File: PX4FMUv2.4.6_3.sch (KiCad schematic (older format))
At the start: 5 parts, among them J301 47346-0001, U302 NUF2042XV6

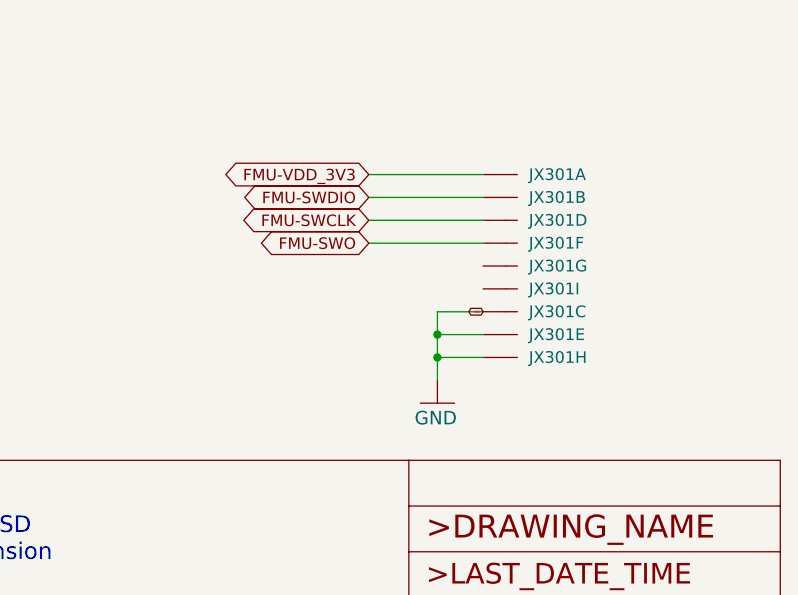
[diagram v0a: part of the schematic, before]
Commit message: removed more things
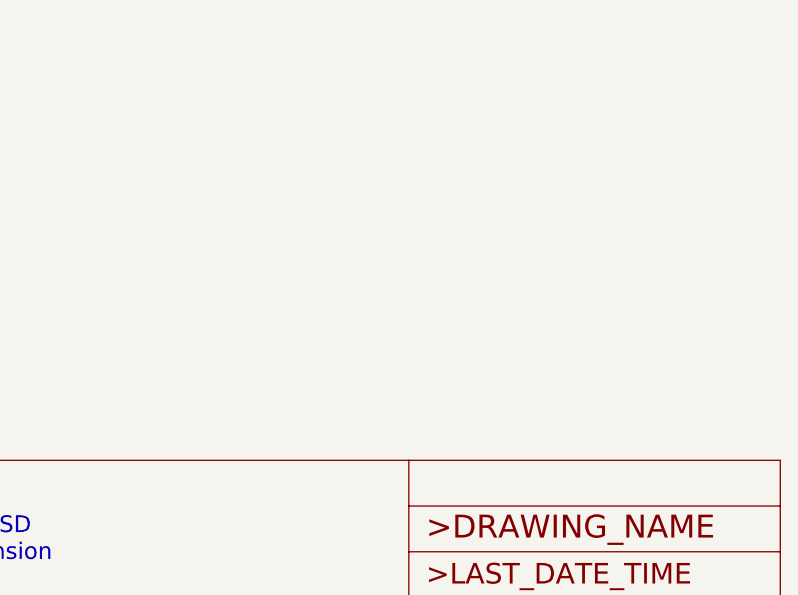
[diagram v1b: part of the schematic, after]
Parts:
- removed JX301: ARM_MINI_JTAG-SMT, PX4FMUv2.4.6:FTSH-105-01-XXX-DV-K, symbol PX4FMUv2.4.6-eagle-import:ARM_MINI_JTAG-SMT
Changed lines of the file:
@@
 $EndDescr
-Wire Wire Line
-	9700 5100 9200 5100
-Text GLabel 9200 5100 0    50   BiDi ~ 0
-FMU-SWDIO
 Wire Wire Line
 	3000 1200 3000 1300
@@
 Text GLabel 4650 1900 0    10   BiDi ~ 0
 GND
-Wire Wire Line
-	9700 5600 9500 5600
-Wire Wire Line
-	9500 5600 9500 5700
-Wire Wire Line
-	9500 5700 9500 5800
-Wire Wire Line
-	9500 5800 9500 5900
-Wire Wire Line
-	9700 5700 9500 5700
-Wire Wire Line
-	9500 5800 9700 5800
-Connection ~ 9500 5700
-Connection ~ 9500 5800
-Text GLabel 9700 5600 0    10   BiDi ~ 0
-GND
-Wire Wire Line
-	9700 5000 9200 5000
-Text GLabel 9200 5000 0    50   BiDi ~ 0
-FMU-VDD_3V3
 Wire Wire Line
 	6600 1200 6800 1200
@@
 Text GLabel 6700 1900 0    50   BiDi ~ 0
 FMU-I2C2_SDA
-Wire Wire Line
-	9700 5300 9200 5300
-Text GLabel 9200 5300 0    50   BiDi ~ 0
-FMU-SWO
-Wire Wire Line
-	9700 5200 9200 5200
-Text GLabel 9200 5200 0    50   BiDi ~ 0
-FMU-SWCLK
 $Comp
 L PX4FMUv2.4.6-eagle-import:A4L-LOC #FRAME6
@@
 	1    0    0    -1
 $EndComp
-$Comp
-L PX4FMUv2.4.6-eagle-import:GND #GND16
-U 1 0 8316678299D4D269
-P 9500 6000
-AR Path="/8316678299D4D269" Ref="#GND16"  Part="1"
-AR Path="/5C109013/8316678299D4D269" Ref="#GND016"  Part="1"
-F 0 "#GND016" H 9500 6000 50  0001 C CNN
-F 1 "GND" H 9400 5900 59  0000 L BNN
-F 2 "" H 9500 6000 50  0001 C CNN
-F 3 "" H 9500 6000 50  0001 C CNN
-	1    9500 6000
-	1    0    0    -1
-$EndComp
-$Comp
-L PX4FMUv2.4.6-eagle-import:ARM_MINI_JTAG-SMT JX301
-U 1 0 F99DB6D9CEB5AE7F
-P 9800 5000
-AR Path="/F99DB6D9CEB5AE7F" Ref="JX301"  Part="1"
-AR Path="/5C109013/F99DB6D9CEB5AE7F" Ref="JX301"  Part="1"
-F 0 "JX301" H 9900 4970 51  0000 L BNN
-F 1 "ARM_MINI_JTAG-SMT" H 9770 5055 59  0001 L BNN
-F 2 "PX4FMUv2.4.6:FTSH-105-01-XXX-DV-K" H 9800 5000 50  0001 C CNN
-F 3 "" H 9800 5000 50  0001 C CNN
-	1    9800 5000
-	1    0    0    -1
-$EndComp
-$Comp
-L PX4FMUv2.4.6-eagle-import:ARM_MINI_JTAG-SMT JX301
-U 2 0 F99DB6D9CEB5AE73
-P 9800 5100
-AR Path="/F99DB6D9CEB5AE73" Ref="JX301"  Part="2"
-AR Path="/5C109013/F99DB6D9CEB5AE73" Ref="JX301"  Part="2"
-F 0 "JX301" H 9900 5070 51  0000 L BNN
-F 1 "ARM_MINI_JTAG-SMT" H 9770 5155 59  0001 L BNN
-F 2 "PX4FMUv2.4.6:FTSH-105-01-XXX-DV-K" H 9800 5100 50  0001 C CNN
-F 3 "" H 9800 5100 50  0001 C CNN
-	2    9800 5100
-	1    0    0    -1
-$EndComp
-$Comp
-L PX4FMUv2.4.6-eagle-import:ARM_MINI_JTAG-SMT JX301
-U 3 0 F99DB6D9CEB5AE77
-P 9800 5600
-AR Path="/F99DB6D9CEB5AE77" Ref="JX301"  Part="3"
-AR Path="/5C109013/F99DB6D9CEB5AE77" Ref="JX301"  Part="3"
-F 0 "JX301" H 9900 5570 51  0000 L BNN
-F 1 "ARM_MINI_JTAG-SMT" H 9770 5655 59  0001 L BNN
-F 2 "PX4FMUv2.4.6:FTSH-105-01-XXX-DV-K" H 9800 5600 50  0001 C CNN
-F 3 "" H 9800 5600 50  0001 C CNN
-	3    9800 5600
-	1    0    0    -1
-$EndComp
-$Comp
-L PX4FMUv2.4.6-eagle-import:ARM_MINI_JTAG-SMT JX301
-U 4 0 F99DB6D9CEB5AE6B
-P 9800 5200
-AR Path="/F99DB6D9CEB5AE6B" Ref="JX301"  Part="4"
-AR Path="/5C109013/F99DB6D9CEB5AE6B" Ref="JX301"  Part="4"
-F 0 "JX301" H 9900 5170 51  0000 L BNN
-F 1 "ARM_MINI_JTAG-SMT" H 9770 5255 59  0001 L BNN
-F 2 "PX4FMUv2.4.6:FTSH-105-01-XXX-DV-K" H 9800 5200 50  0001 C CNN
-F 3 "" H 9800 5200 50  0001 C CNN
-	4    9800 5200
-	1    0    0    -1
-$EndComp
-$Comp
-L PX4FMUv2.4.6-eagle-import:ARM_MINI_JTAG-SMT JX301
-U 5 0 F99DB6D9CEB5AE6F
-P 9800 5700
-AR Path="/F99DB6D9CEB5AE6F" Ref="JX301"  Part="5"
-AR Path="/5C109013/F99DB6D9CEB5AE6F" Ref="JX301"  Part="5"
-F 0 "JX301" H 9900 5670 51  0000 L BNN
-F 1 "ARM_MINI_JTAG-SMT" H 9770 5755 59  0001 L BNN
-F 2 "PX4FMUv2.4.6:FTSH-105-01-XXX-DV-K" H 9800 5700 50  0001 C CNN
-F 3 "" H 9800 5700 50  0001 C CNN
-	5    9800 5700
-	1    0    0    -1
-$EndComp
-$Comp
-L PX4FMUv2.4.6-eagle-import:ARM_MINI_JTAG-SMT JX301
-U 6 0 F99DB6D9CEB5AE63
-P 9800 5300
-AR Path="/F99DB6D9CEB5AE63" Ref="JX301"  Part="6"
-AR Path="/5C109013/F99DB6D9CEB5AE63" Ref="JX301"  Part="6"
-F 0 "JX301" H 9900 5270 51  0000 L BNN
-F 1 "ARM_MINI_JTAG-SMT" H 9770 5355 59  0001 L BNN
-F 2 "PX4FMUv2.4.6:FTSH-105-01-XXX-DV-K" H 9800 5300 50  0001 C CNN
-F 3 "" H 9800 5300 50  0001 C CNN
-	6    9800 5300
-	1    0    0    -1
-$EndComp
-$Comp
-L PX4FMUv2.4.6-eagle-import:ARM_MINI_JTAG-SMT JX301
-U 7 0 F99DB6D9CEB5AE67
-P 9800 5400
-AR Path="/F99DB6D9CEB5AE67" Ref="JX301"  Part="7"
-AR Path="/5C109013/F99DB6D9CEB5AE67" Ref="JX301"  Part="7"
-F 0 "JX301" H 9900 5370 51  0000 L BNN
-F 1 "ARM_MINI_JTAG-SMT" H 9770 5455 59  0001 L BNN
-F 2 "PX4FMUv2.4.6:FTSH-105-01-XXX-DV-K" H 9800 5400 50  0001 C CNN
-F 3 "" H 9800 5400 50  0001 C CNN
-	7    9800 5400
-	1    0    0    -1
-$EndComp
-$Comp
-L PX4FMUv2.4.6-eagle-import:ARM_MINI_JTAG-SMT JX301
-U 8 0 F99DB6D9CEB5AE5B
-P 9800 5800
-AR Path="/F99DB6D9CEB5AE5B" Ref="JX301"  Part="8"
-AR Path="/5C109013/F99DB6D9CEB5AE5B" Ref="JX301"  Part="8"
-F 0 "JX301" H 9900 5770 51  0000 L BNN
-F 1 "ARM_MINI_JTAG-SMT" H 9770 5855 59  0001 L BNN
-F 2 "PX4FMUv2.4.6:FTSH-105-01-XXX-DV-K" H 9800 5800 50  0001 C CNN
-F 3 "" H 9800 5800 50  0001 C CNN
-	8    9800 5800
-	1    0    0    -1
-$EndComp
-$Comp
-L PX4FMUv2.4.6-eagle-import:ARM_MINI_JTAG-SMT JX301
-U 9 0 F99DB6D9CEB5AE5F
-P 9800 5500
-AR Path="/F99DB6D9CEB5AE5F" Ref="JX301"  Part="9"
-AR Path="/5C109013/F99DB6D9CEB5AE5F" Ref="JX301"  Part="9"
-F 0 "JX301" H 9900 5470 51  0000 L BNN
-F 1 "ARM_MINI_JTAG-SMT" H 9770 5555 59  0001 L BNN
-F 2 "PX4FMUv2.4.6:FTSH-105-01-XXX-DV-K" H 9800 5500 50  0001 C CNN
-F 3 "" H 9800 5500 50  0001 C CNN
-	9    9800 5500
-	1    0    0    -1
-$EndComp
